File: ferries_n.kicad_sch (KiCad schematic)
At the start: 4 parts

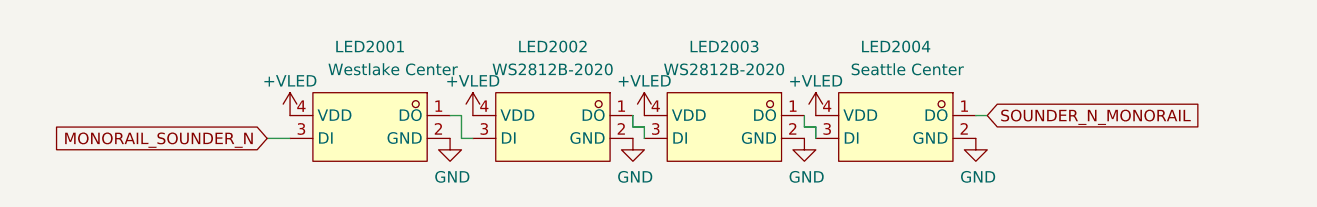
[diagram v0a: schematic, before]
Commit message: rev-b validation run
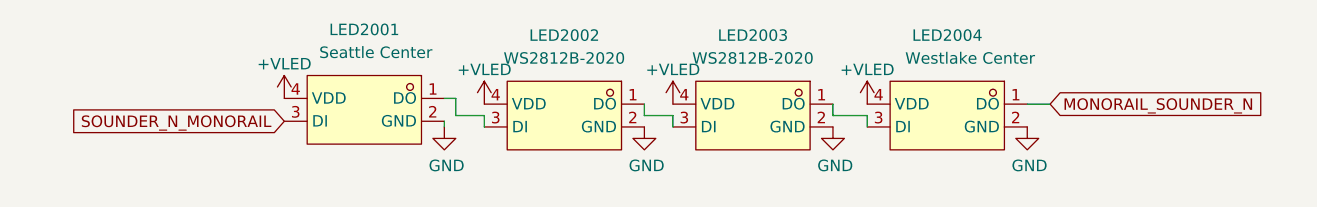
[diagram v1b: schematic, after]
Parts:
- LED2001: LCSC Part C965555 -> C52917434; Monorail Westlake Center -> Seattle Center
- LED2002, LED2003: LCSC Part C965555 -> C52917434
- LED2004: LCSC Part C965555 -> C52917434; Monorail Seattle Center -> Westlake Center
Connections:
- net MONORAIL_SOUNDER_N: now also LED2004.1 (DO); no longer LED2001.3 (DI)
- net SOUNDER_N_MONORAIL: now also LED2001.3 (DI); no longer LED2004.1 (DO)
